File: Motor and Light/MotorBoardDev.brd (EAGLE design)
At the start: 93.5 x 80.5 mm, 88 parts, among them J1 Under Glow, J2 Safety Light, J3 12V, J4 24V, Q1 TIP42C, Q10 TIP42C, Q11 TIP42C, Q15 TIP41C, Q16 TIP41C, Q2 220mA/50V/3.5Ω, Q3 TIP42C, Q4 TIP42C, Q5 TIP42C, Q6 TIP42C, Q7 220mA/50V/3.5Ω, Q8 220mA/50V/3.5Ω, Q9 220mA/50V/3.5Ω, T1 NCP1117DT50GOS-ND, T2 TIP41A, T3 NCP1117DT33GOS-ND, U2 9DoF IMU, X1 C-GRID-05-15-91, X2 C-GRID-05-15-91, X3 MINI-USB_SHIELD5P4-32005-400, X4 C-GRID-02-70553, X5 SI-50170, X7 2510-, X8 2510-

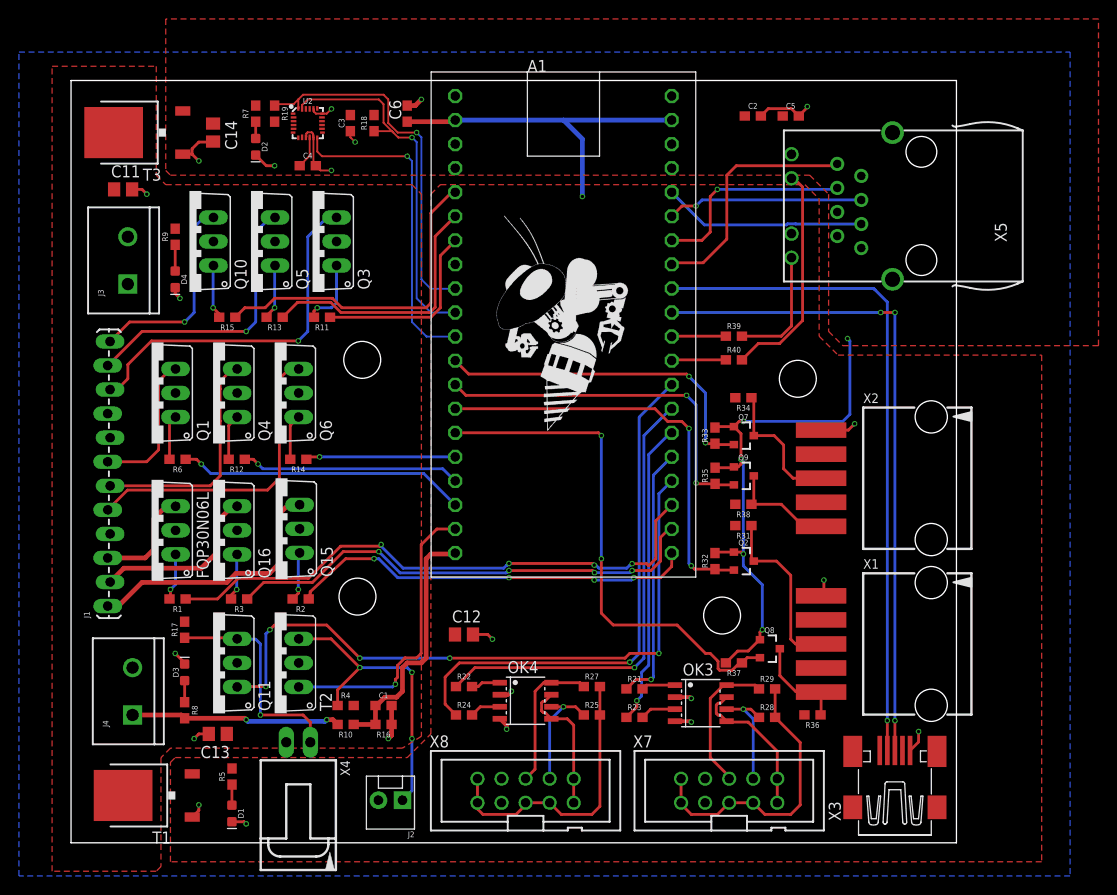
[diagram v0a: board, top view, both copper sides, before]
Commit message: Before Review
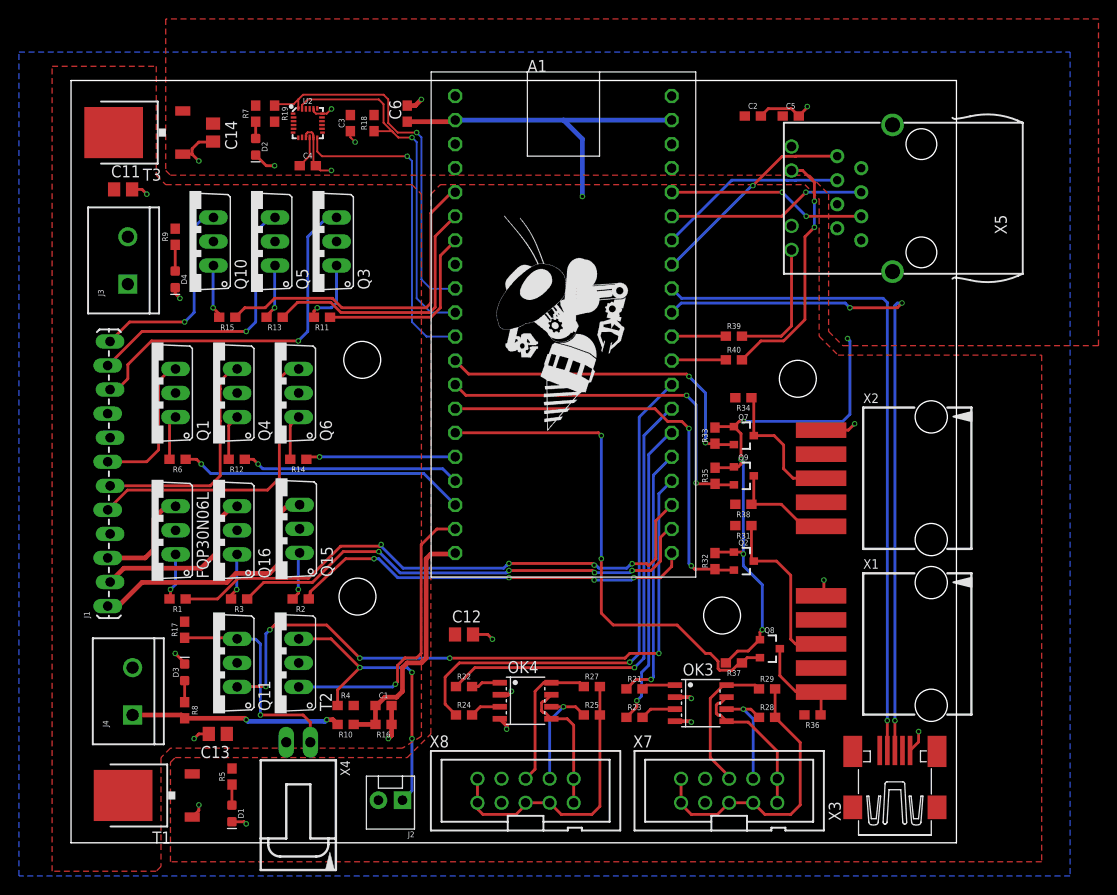
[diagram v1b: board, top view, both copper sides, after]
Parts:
- moved X5 0.81 mm to (86.8, 68.1)
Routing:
- net TD+: track 25.8 -> 22.2 mm, vias 0 -> 1
- net D+: track 69.8 -> 73.0 mm
- net ETH_LED2: track 23.8 -> 26.3 mm, vias 0 -> 2
- net TD-: track 22.0 -> 20.1 mm, vias 1 -> 0
- net ETH_LED1: track 12.9 -> 13.7 mm
- net RD-: track 21.5 -> 21.1 mm, vias 0 -> 2
